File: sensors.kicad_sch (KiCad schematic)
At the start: 8 parts, among them U3 ICM-42688-P, U5 MCP98243, U6 MCP98243

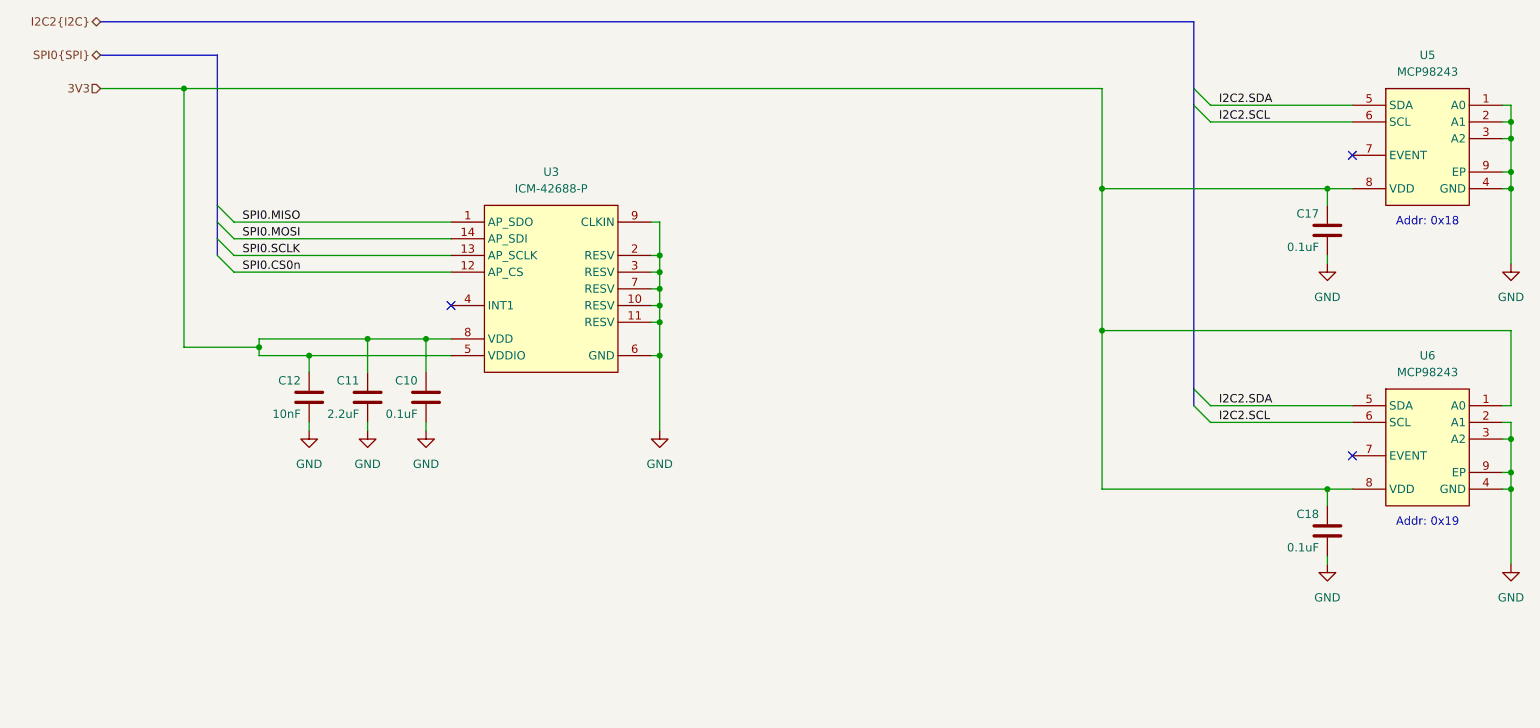
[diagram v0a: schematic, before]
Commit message: finished defining spi/i2c gpio, CAN, off-board signals
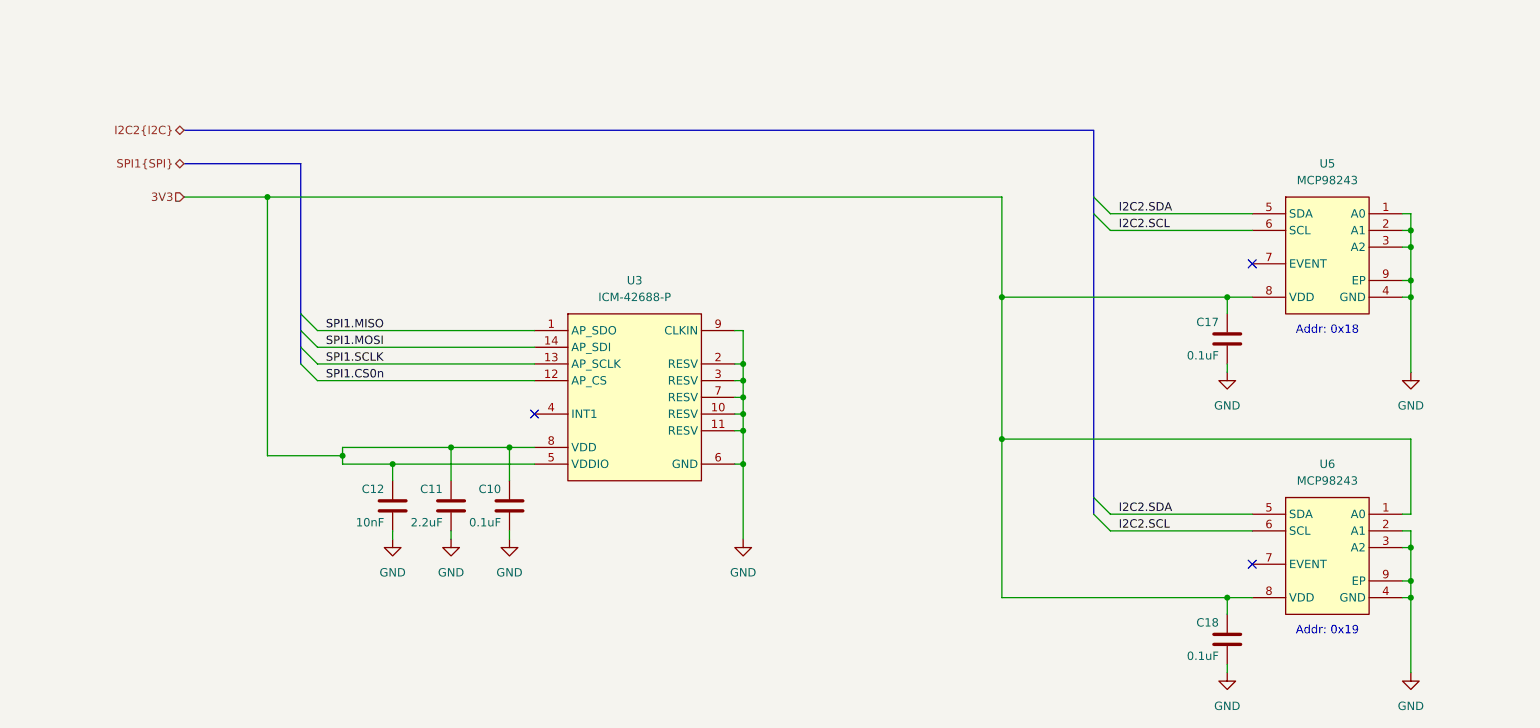
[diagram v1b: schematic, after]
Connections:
- net SPI0.CS0n renamed SPI1.CS0n
- net SPI0.MISO renamed SPI1.MISO
- net SPI0.MOSI renamed SPI1.MOSI
- net SPI0.SCLK renamed SPI1.SCLK
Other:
- moved on the sheet: C10, C11, C12, C17, C18, U3, U5, U6
